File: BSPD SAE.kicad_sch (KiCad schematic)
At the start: 62 parts, among them Q1 MMBT3904, Q2 2N7002K, Q3 MMBT3904, U1 LTC6994xS6-2, U2 TPS7A2501DRVR, U3 TLV1824, U4 TLV1824

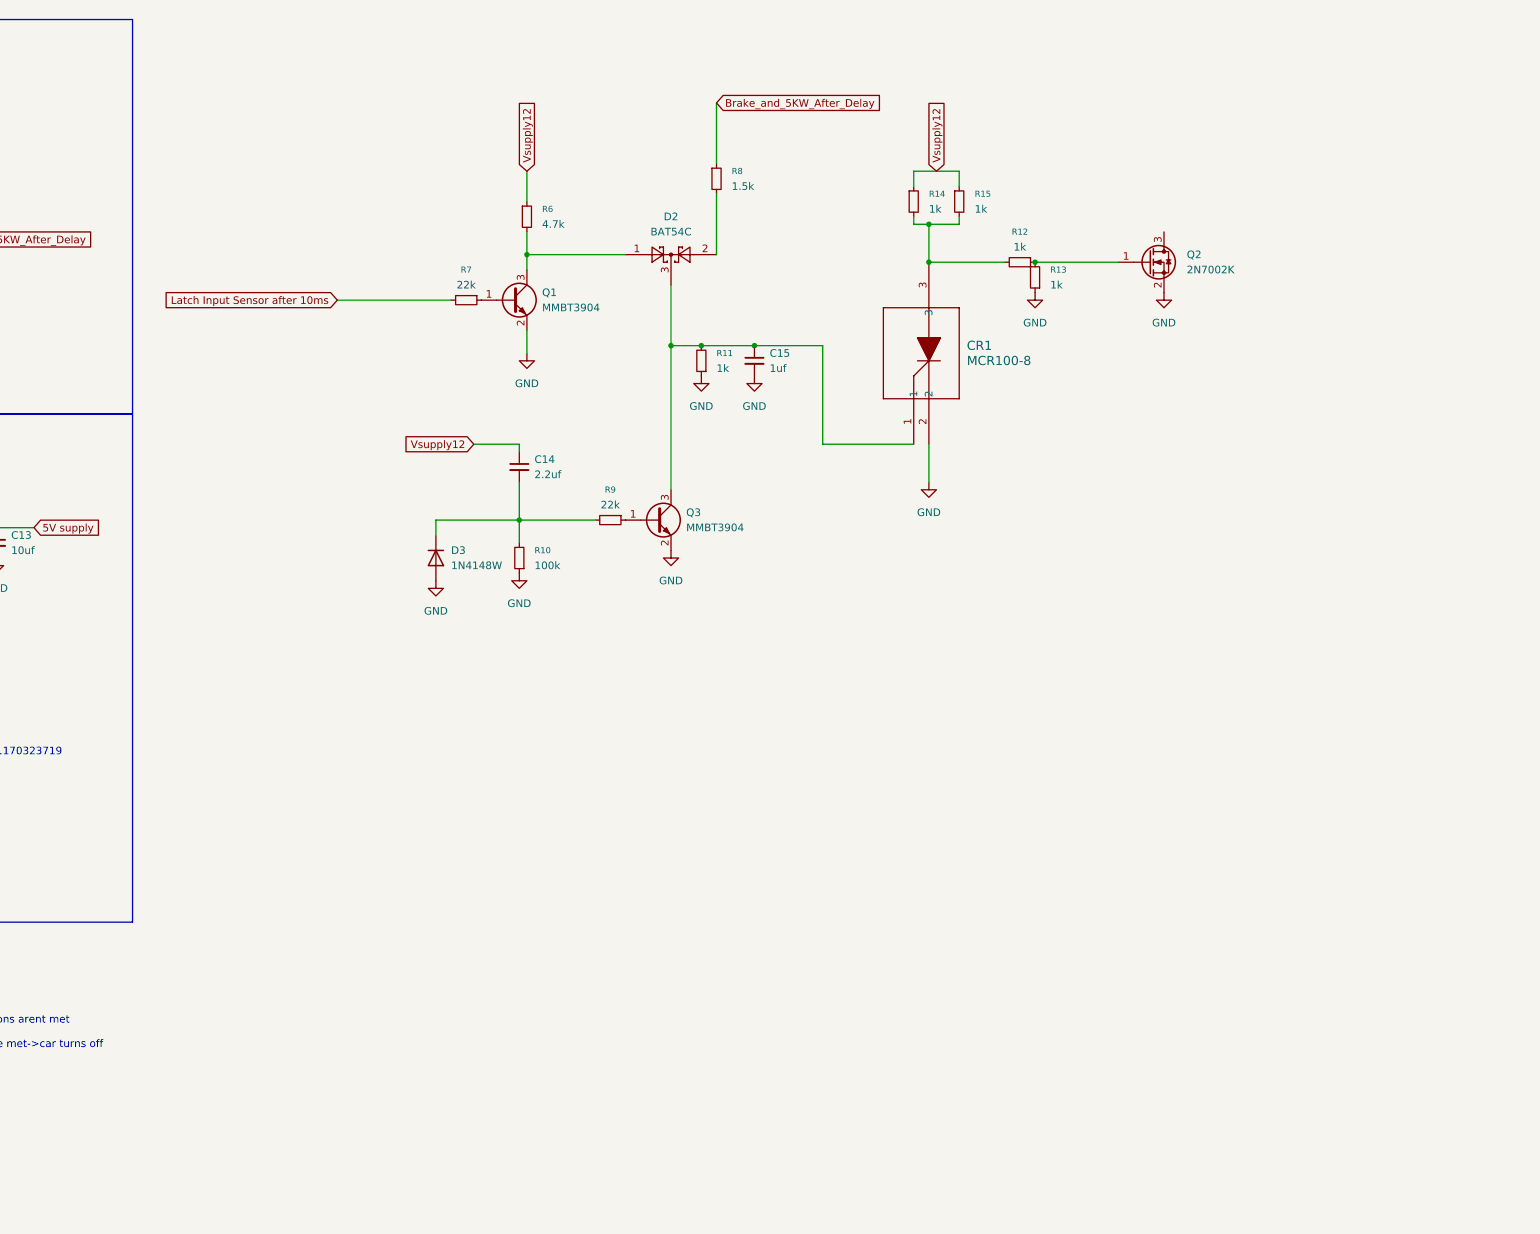
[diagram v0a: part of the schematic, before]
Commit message: autosave 2026-10-05 00:11:05
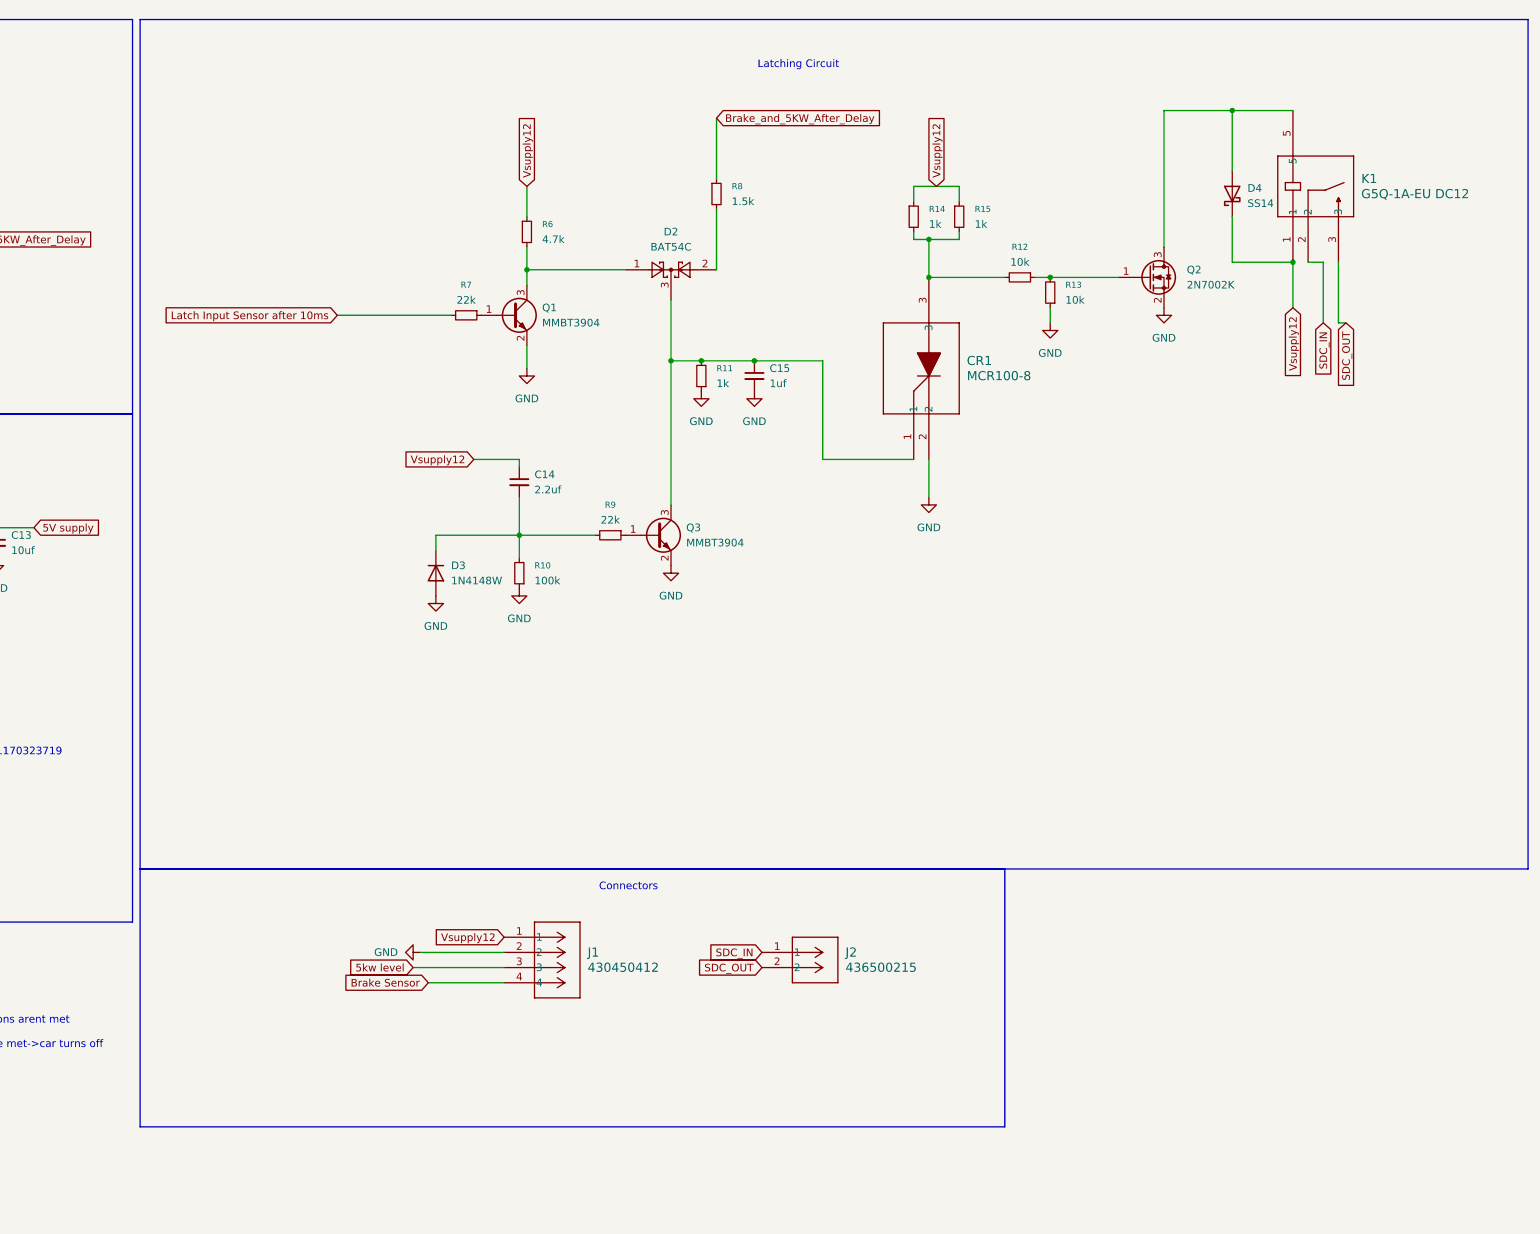
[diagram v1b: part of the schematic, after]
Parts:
- added D4: SS14, Diode_SMD:D_SMA, symbol Diode:SS14
- added J1: 430450412, CONN_SD-43045-005_04_MOL, symbol 2026-10-05_06-33-49:430450412
- added J2: 436500215, CONN_SD-43650-006_02_MOL, symbol 2026-10-05_06-36-43:436500215
- added K1: G5Q-1A-EU DC12, RELAY_G5Q-1A DC5_OMR, symbol 2026-10-05_06-05-09:G5Q-1A-EU_DC12
- R12, R13: value 1k -> 10k
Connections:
- net 5kw level: now also J1.3
- net Brake Sensor: now also J1.4
- net GND: now also J1.2
- net Vsupply12: now also D4.1 (K), J1.1, K1.1
- net at Q2.3 (D): now also D4.2 (A), K1.5
- new net SDC_IN: J2.1, K1.2
- new net SDC_OUT: J2.2, K1.3
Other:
- note added: "Connectors"
- note added: "Latching Circuit"
- moved on the sheet: C14, C15, CR1, D2, D3, Q1, Q2, Q3, R10, R11, R12, R13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
